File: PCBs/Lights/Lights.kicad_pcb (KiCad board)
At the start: 2 copper layers, 6 parts, among them J1 Conn_01x02

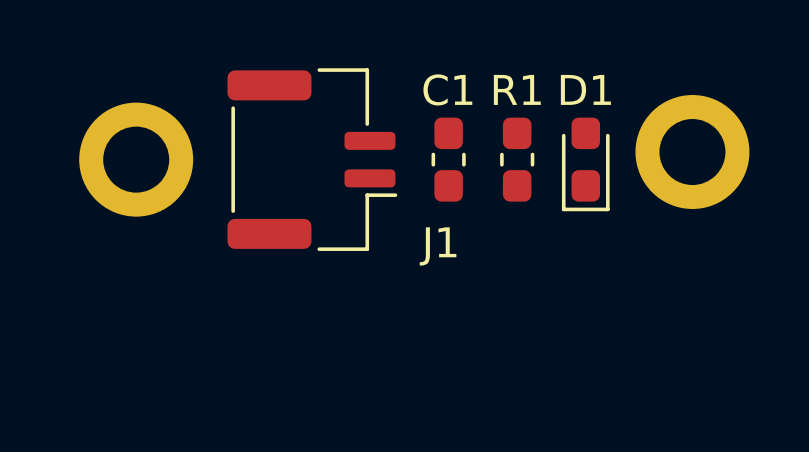
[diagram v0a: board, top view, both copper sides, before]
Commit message: board complete
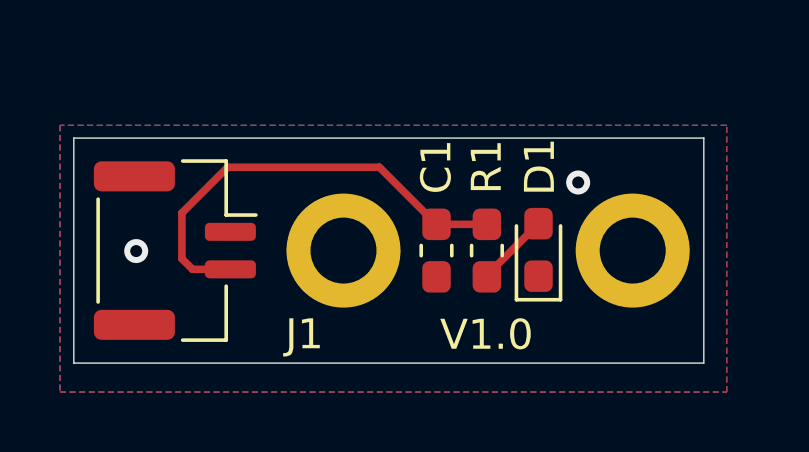
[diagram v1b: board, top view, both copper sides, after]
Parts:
- J1: footprint Connector_JST:JST_GH_BM02B-GHS-TBT_1x02-1MP_P1.25mm_Vertical -> Connector_JST:JST_GH_SM02B-GHS-TB_1x02-1MP_P1.25mm_Horizontal
- moved H1 7.55 mm to (139.0, 96.2)
- moved J1 5.47 mm to (133.4, 96.2), turned to 270 degrees
- moved H2 3.84 mm to (148.6, 96.2)
- moved D1 3.40 mm to (145.5, 96.2)
- moved R1 3.20 mm to (143.8, 96.2)
- moved C1 3.06 mm to (142.1, 96.2)
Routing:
- net +5V: track 0.00 -> 14.9 mm
- net Net-(D1-Pad2): track 0.00 -> 2.48 mm
- net GND: vias 0 -> 2
- added copper zone on B.Cu, net GND
- added copper zone on F.Cu, net GND
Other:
- board outline added: 21 x 7.5 mm
- net class Default: clearance 0.2 -> 0.1778; trace_width 0.25 -> 0.254
- rule trace_clearance: 0.2 -> 0.1778
- board text added: "V1.0"
